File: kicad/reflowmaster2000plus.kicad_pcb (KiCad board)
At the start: 2 copper layers, 48.8 x 24.1 mm, 21 parts, among them IC1 TLP3036, P1 CONN_8, P2 Toaster, P3 220V, U1 TRIAC, U2 TLC2272

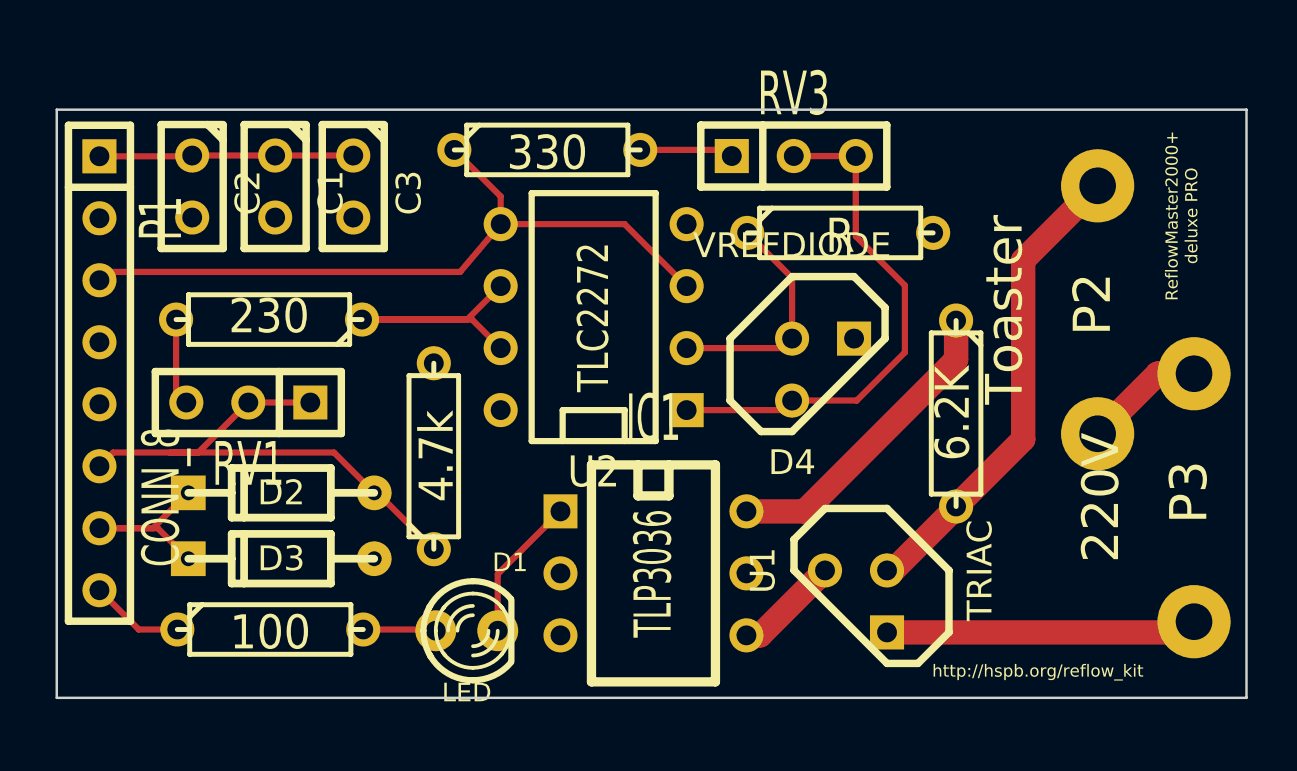
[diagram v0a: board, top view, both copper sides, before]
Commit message: [enh] lot's of polishing
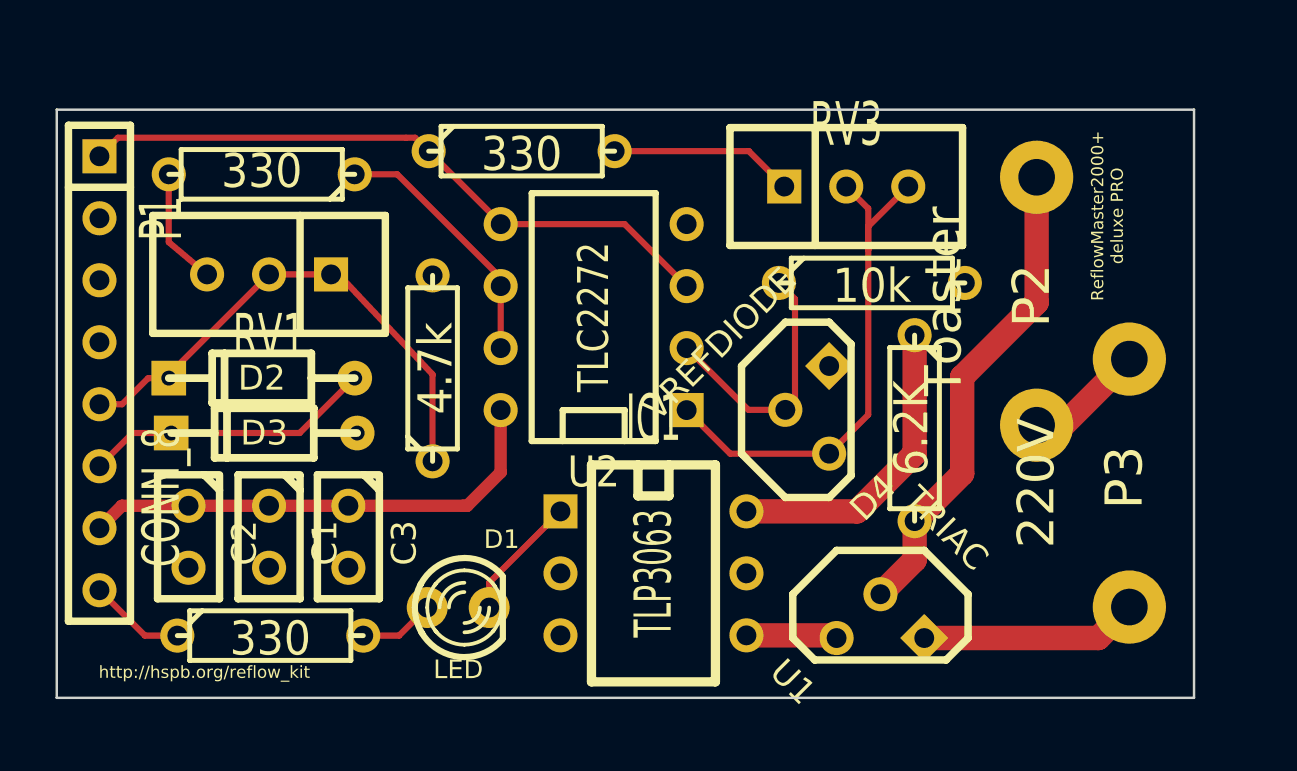
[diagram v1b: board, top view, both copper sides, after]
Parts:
- C1: value C -> 10u
- C2: value C -> 100n
- C3: value C -> 10n
- IC1: value TLP3036 -> TLP3063
- R2: value 230 -> 330
- R4: value 100 -> 330
- R6: value R -> 10k
- RV1, RV3: value POT -> 500
- moved C1 14.4 mm to (163.8, 136.7)
- moved C3 14.4 mm to (167.1, 136.7)
- moved C2 14.4 mm to (160.5, 136.7)
- moved R2 5.96 mm to (163.5, 121.8)
- moved RV1 5.32 mm to (163.8, 126.0)
- moved D3 5.20 mm to (163.6, 132.4)
- moved D2 4.77 mm to (163.5, 130.2)
- moved R5 3.60 mm to (170.5, 129.8)
- moved P3 2.72 mm to (199.1, 134.5)
- moved P2 2.52 mm to (195.2, 127.0)
- moved RV3 2.49 mm to (187.4, 122.3)
- moved R6 2.43 mm to (188.5, 126.3)
- moved U1 1.80 mm to (188.8, 140.8), turned to 315 degrees
- moved R1 1.80 mm to (190.2, 132.2)
- moved D4 1.67 mm to (186.8, 131.5), turned to 45 degrees
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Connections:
- net AGND renamed GNDPWR
- C1 pad 1: /+12V -> +12V
- C2 pad 1: /+12V -> +12V
- C3 pad 1: /+12V -> +12V
- D2 pad 1: /Utemp -> /Uclamp
- D2 pad 2: /Uclamp -> /Utemp
- P1 pad 1: /+12V -> /KTYa
- P1 pad 3: /KTYa -> GND
- P1 pad 5: GND -> /Utemp
- P1 pad 6: /Utemp -> /Uclamp
- P1 pad 7: /Uclamp -> +12V
- U2 pad 4: (no net) -> GND
- U2 pad 8: (no net) -> +12V
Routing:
- net +12V: track 0.00 -> 19.9 mm
- net /+12V: track 10.4 -> 0.00 mm
- net N-000009: track 13.4 -> 8.93 mm
- net N-0000018: track 3.85 -> 7.55 mm
- net /Uclamp: track 8.40 -> 12.0 mm
- net /KTYa: track 30.0 -> 26.9 mm
- net N-000007: track 12.4 -> 10.6 mm
- net GNDPWR: track 6.46 -> 4.92 mm
- net N-0000012: track 3.57 -> 4.83 mm
- net N-000003: track 9.57 -> 10.7 mm
- net /Utemp: track 22.2 -> 21.3 mm
- net N-000002: track 5.95 -> 5.15 mm
- net N-0000011: track 4.36 -> 3.74 mm
- net N-0000016: track 21.3 -> 21.8 mm
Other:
- board size 48.8 x 24.1 mm -> 46.6 x 24.1 mm
